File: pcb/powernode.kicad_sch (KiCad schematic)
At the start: 11 parts, among them Q2 2SC1623 300-400, Q4 IRLML6402

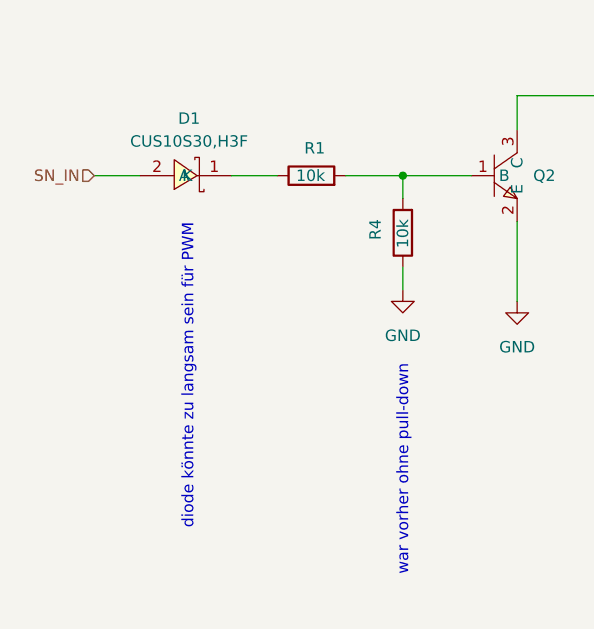
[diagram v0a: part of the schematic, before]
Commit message: dienstag
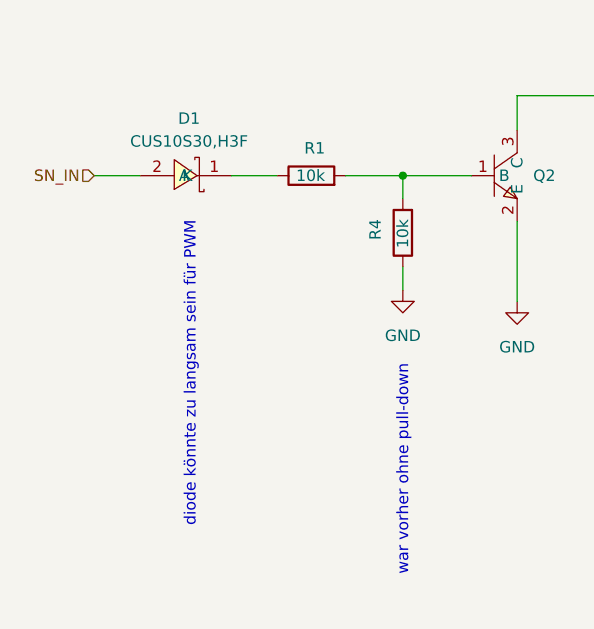
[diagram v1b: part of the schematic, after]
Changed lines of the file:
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@@
 	(text "diode könnte zu langsam sein für PWM"
 		(exclude_from_sim no)
-		(at 77.724 120.142 90)
+		(at 77.978 119.888 90)
 		(effects
 			(font
